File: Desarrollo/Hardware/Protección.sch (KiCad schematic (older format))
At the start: 46 parts, among them J1 Entradas Analógicas, U1 TPD2E001, U2 TPD2E001, U3 TPD2E001, U4 TPD2E001, U5 TPD2E001, U6 TPD2E001, U7 TPD2E001, U8 TPD2E001, U9 TPD2E001

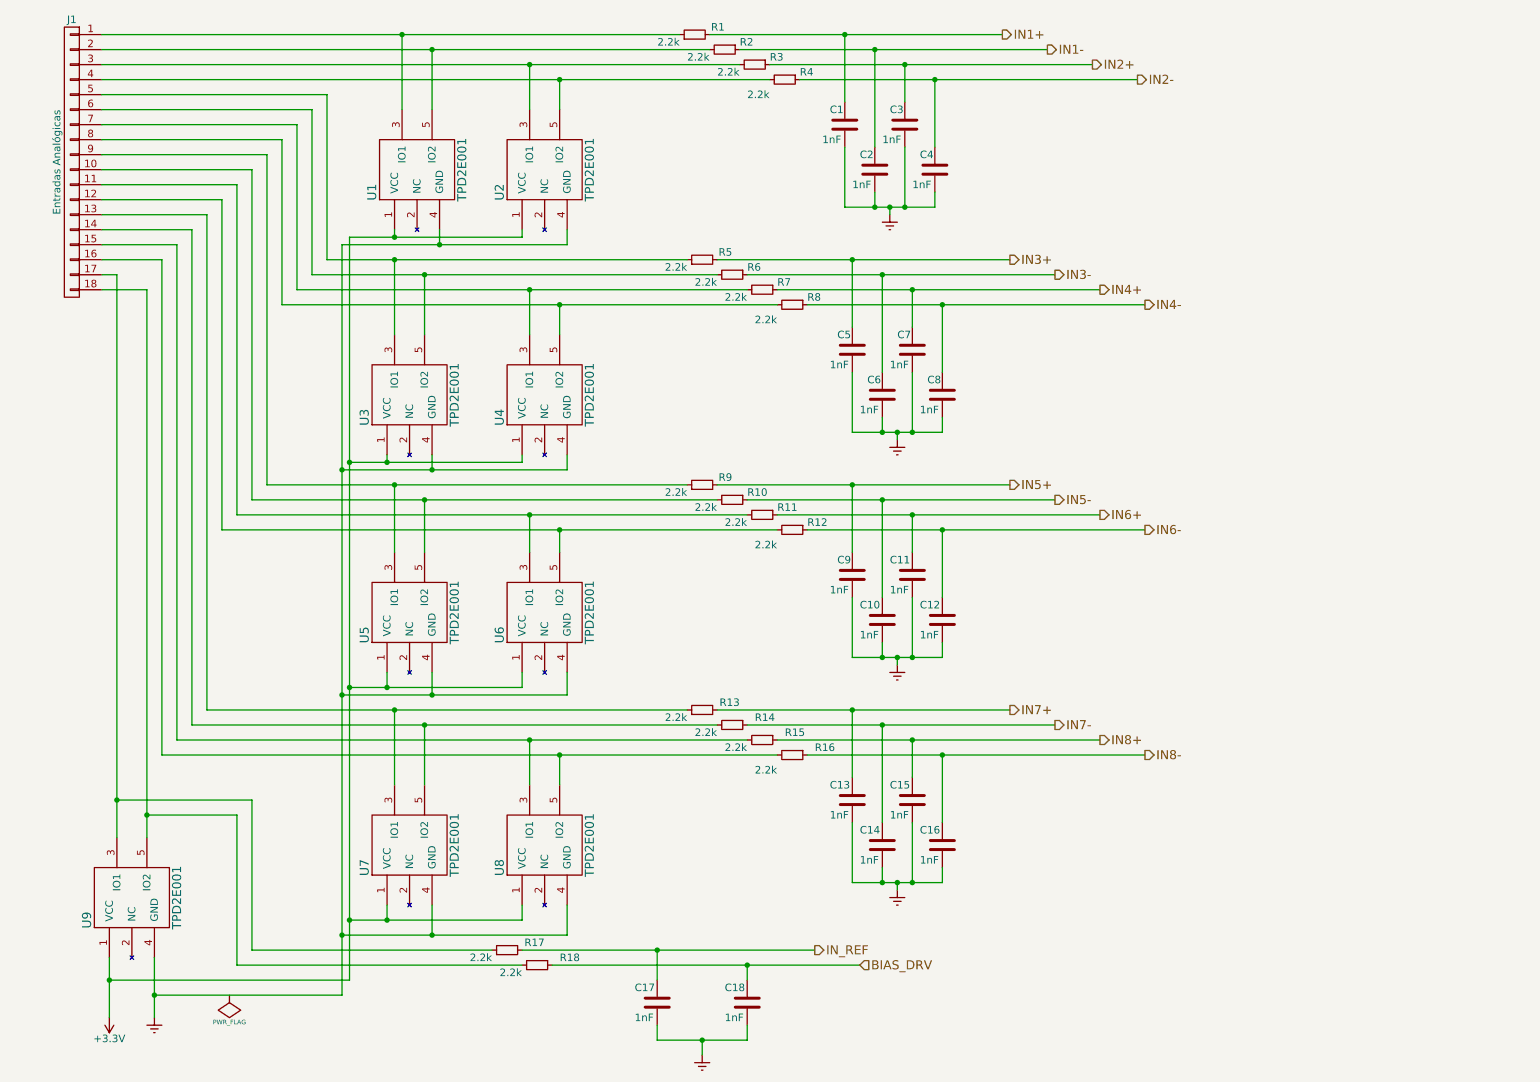
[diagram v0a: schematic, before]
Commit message: Finalización de primer ruteo estimado. Revisión de cantidad de v
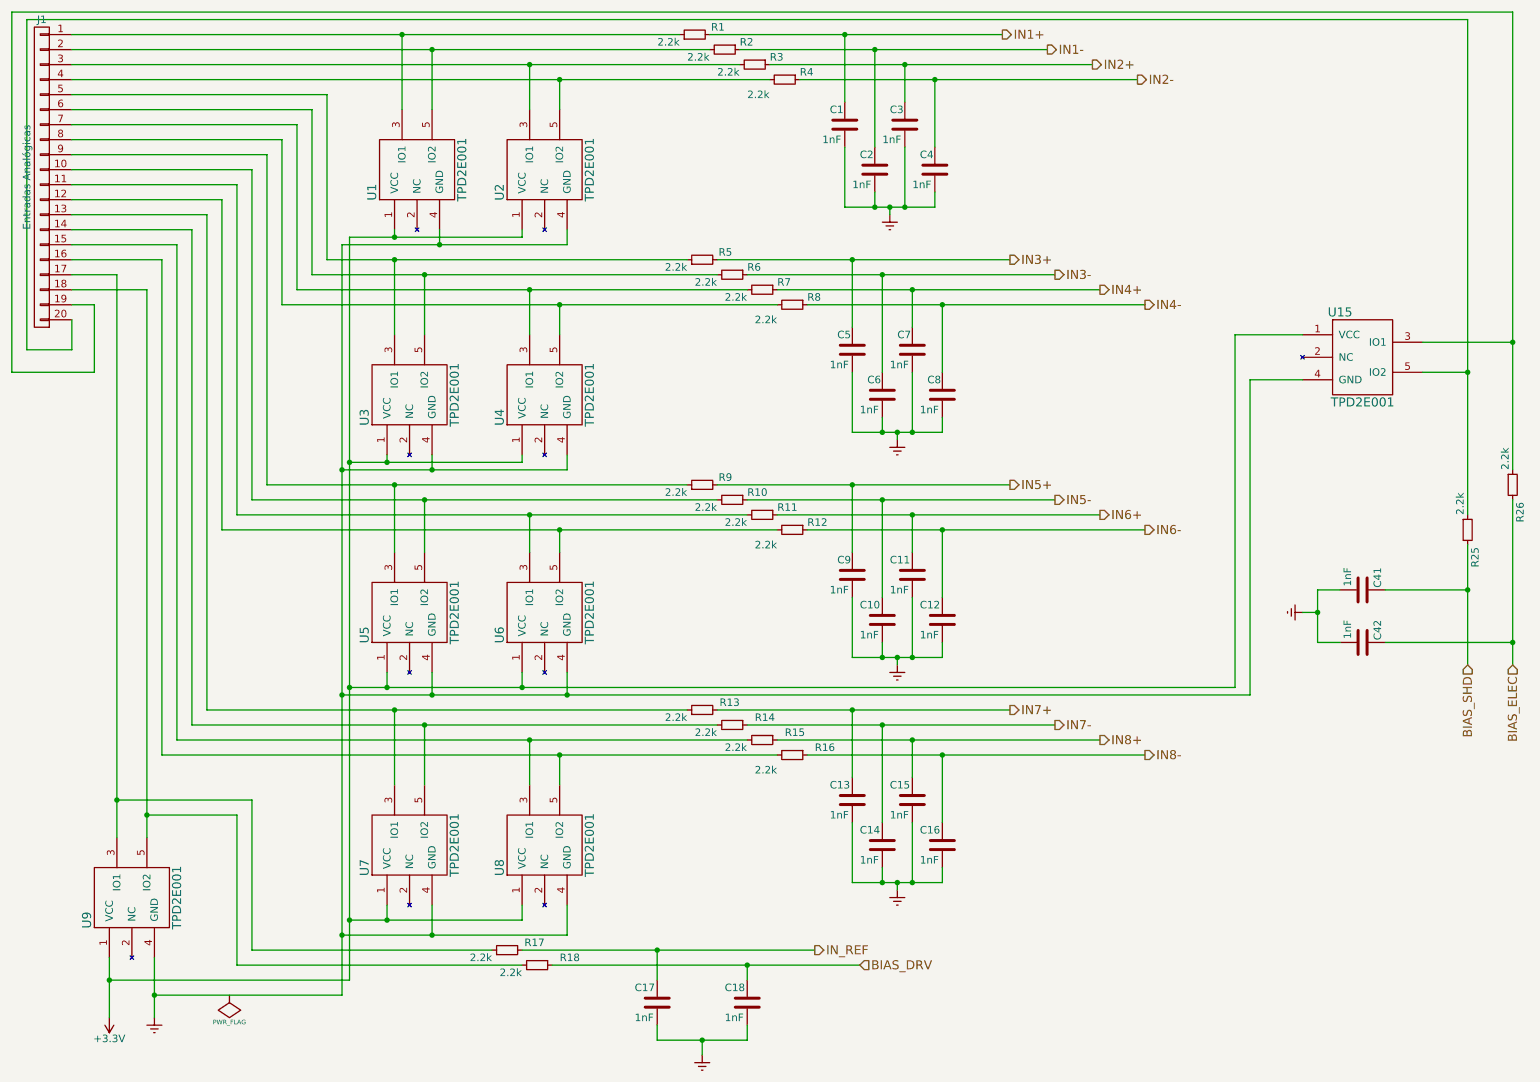
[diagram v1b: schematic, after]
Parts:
- removed J1: Entradas Analógicas, Pin_Headers:Pin_Header_Straight_1x18, symbol CONN_01X18
- added C41, C42: 1nF, Capacitors_SMD:C_0805, symbol C
- added J1: Entradas Analógicas, Pin_Headers:Pin_Header_Straight_1x20, symbol CONN_01X20
- added R25, R26: 2.2k, Resistors_SMD:R_0805, symbol R_Small
- added U15: TPD2E001, TO_SOT_Packages_SMD:SOT-23-5, symbol TPD2E001
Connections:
- net +3V3: now also U15.1 (VCC)
- net Earth: now also C41.2, C42.2, U15.4 (GND)
- net at R1.1, U1.3 (IO1): now also J1.1 (P1)
- net at R10.2, U5.5 (IO2): now also J1.10 (P10)
- net at R11.2, U6.3 (IO1): now also J1.11 (P11)
- net at R12.2, U6.5 (IO2): now also J1.12 (P12)
- net at R13.1, U7.3 (IO1): now also J1.13 (P13)
- net at R14.2, U7.5 (IO2): now also J1.14 (P14)
- net at R15.2, U8.3 (IO1): now also J1.15 (P15)
- net at R16.2, U8.5 (IO2): now also J1.16 (P16)
- net at R17.1, U9.3 (IO1): now also J1.17 (P17)
- net at R18.2, U9.5 (IO2): now also J1.18 (P18)
- net at R2.2, U1.5 (IO2): now also J1.2 (P2)
- net at R3.2, U2.3 (IO1): now also J1.3 (P3)
- net at R4.2, U2.5 (IO2): now also J1.4 (P4)
- net at R5.1, U3.3 (IO1): now also J1.5 (P5)
- net at R6.2, U3.5 (IO2): now also J1.6 (P6)
- net at R7.2, U4.3 (IO1): now also J1.7 (P7)
- net at R8.2, U4.5 (IO2): now also J1.8 (P8)
- net at R9.1, U5.3 (IO1): now also J1.9 (P9)
- new net: J1.19 (P19), R26.1, U15.3 (IO1)
- new net: J1.20 (P20), R25.1, U15.5 (IO2)
- new net BIAS_ELEC: C42.1, R26.2
- new net BIAS_SHD: C41.1, R25.2
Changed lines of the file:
@@
 encoding utf-8
 Sheet 2 4
-Title ""
+Title "Entradas Analógicas y Protección"
 Date ""
-Rev ""
-Comp ""
+Rev "1.0"
+Comp "Bruno Javier Cesario"
 Comment1 ""
 Comment2 ""
@@
 Comment4 ""
 $EndDescr
-$Comp
-L CONN_01X18 J1
-U 1 1 57BF0F9F
-P 950 1550
-F 0 "J1" H 950 2500 50  0000 C CNN
-F 1 "Entradas Analógicas" V 1050 1550 50  0000 C CNN
-F 2 "Pin_Headers:Pin_Header_Straight_1x18" H 950 1550 50  0001 C CNN
-F 3 "" H 950 1550 50  0000 C CNN
-	1    950  1550
-	-1   0    0    -1
-$EndComp
 $Comp
 L R_Small R1
@@
 $EndComp
 Wire Wire Line
-	2650 2200 2650 1100
-Wire Wire Line
-	2650 1100 1150 1100
-Wire Wire Line
-	1150 1200 2550 1200
+	2650 1100 2650 2200
+Wire Wire Line
+	950  1100 2650 1100
+Wire Wire Line
+	950  1200 2550 1200
 Wire Wire Line
 	2550 1200 2550 2300
 Wire Wire Line
-	2450 2400 2450 1300
-Wire Wire Line
-	2450 1300 1150 1300
-Wire Wire Line
-	1150 1400 2350 1400
+	2450 1300 2450 2400
+Wire Wire Line
+	950  1300 2450 1300
+Wire Wire Line
+	950  1400 2350 1400
 Wire Wire Line
 	2350 1400 2350 2500
 Wire Wire Line
-	1150 1500 2250 1500
+	950  1500 2250 1500
 Wire Wire Line
 	2250 1500 2250 3700
 Wire Wire Line
-	2150 3800 2150 1600
-Wire Wire Line
-	2150 1600 1150 1600
-Wire Wire Line
-	1150 1700 2050 1700
+	2150 1600 2150 3800
+Wire Wire Line
+	950  1600 2150 1600
+Wire Wire Line
+	950  1700 2050 1700
 Wire Wire Line
 	2050 1700 2050 3900
 Wire Wire Line
-	1950 4000 1950 1800
-Wire Wire Line
-	1950 1800 1150 1800
+	1950 1800 1950 4000
+Wire Wire Line
+	950  1800 1950 1800
 Wire Wire Line
 	1850 1900 1850 5200
 Wire Wire Line
-	1850 1900 1150 1900
-Wire Wire Line
-	1150 2000 1750 2000
+	950  1900 1850 1900
+Wire Wire Line
+	950  2000 1750 2000
 Wire Wire Line
 	1750 2000 1750 5300
@@
 	1650 2100 1650 5400
 Wire Wire Line
-	1650 2100 1150 2100
-Wire Wire Line
-	1150 2200 1550 2200
+	950  2100 1650 2100
+Wire Wire Line
+	950  2200 1550 2200
 Wire Wire Line
 	1550 2200 1550 5500
 Wire Wire Line
-	1150 2300 1250 2300
+	950  2300 1250 2300
 Wire Wire Line
 	1250 2300 1250 6050
 Wire Wire Line
-	1150 2400 1450 2400
+	950  2400 1450 2400
 Wire Wire Line
 	1450 2400 1450 6050
@@
 Connection ~ 5150 7400
 Wire Wire Line
-	1150 700  5000 700
-Wire Wire Line
-	1150 800  5200 800
-Wire Wire Line
-	1150 900  5400 900
-Wire Wire Line
-	1150 1000 5600 1000
+	950  700  5000 700
+Wire Wire Line
+	950  800  5200 800
+Wire Wire Line
+	950  900  5400 900
+Wire Wire Line
+	950  1000 5600 1000
 Wire Wire Line
 	3150 1200 3150 700
@@
 	3050 4950 3050 5050
 Wire Wire Line
-	2800 5050 3950 5050
+	2800 5050 8700 5050
 Wire Wire Line
 	3950 5050 3950 4950
@@
 	3350 4950 3350 5100
 Wire Wire Line
-	2750 5100 4250 5100
+	2750 5100 8800 5100
 Wire Wire Line
 	4250 5100 4250 4950
@@
 	-1   0    0    1
 $EndComp
+$Comp
+L TPD2E001 U15
+U 1 1 57D06AC4
+P 9550 2850
+F 0 "U15" H 9400 3150 60  0000 C CNN
+F 1 "TPD2E001" H 9550 2550 60  0000 C CNN
+F 2 "TO_SOT_Packages_SMD:SOT-23-5" H 9550 2850 60  0001 C CNN
+F 3 "" H 9550 2850 60  0000 C CNN
+	1    9550 2850
+	1    0    0    -1
+$EndComp
+$Comp
+L R_Small R26
+U 1 1 57D06E46
+P 10550 3700
+F 0 "R26" V 10600 3450 50  0000 L CNN
+F 1 "2.2k" V 10500 3800 50  0000 L CNN
+F 2 "Resistors_SMD:R_0805" H 10550 3700 50  0001 C CNN
+F 3 "" H 10550 3700 50  0000 C CNN
+	1    10550 3700
+	1    0    0    -1
+$EndComp
+$Comp
+L R_Small R25
+U 1 1 57D0710C
+P 10250 4000
+F 0 "R25" V 10300 3750 50  0000 L CNN
+F 1 "2.2k" V 10200 4100 50  0000 L CNN
+F 2 "Resistors_SMD:R_0805" H 10250 4000 50  0001 C CNN
+F 3 "" H 10250 4000 50  0000 C CNN
+	1    10250 4000
+	1    0    0    -1
+$EndComp
+$Comp
+L C C41
+U 1 1 57D079C5
+P 9550 4400
+F 0 "C41" H 9400 4500 50  0000 L CNN
+F 1 "1nF" H 9400 4300 50  0000 L CNN
+F 2 "Capacitors_SMD:C_0805" H 9588 4250 50  0001 C CNN
+F 3 "" H 9550 4400 50  0000 C CNN
+	1    9550 4400
+	0    1    1    0
+$EndComp
+$Comp
+L C C42
+U 1 1 57D07AE3
+P 9550 4750
+F 0 "C42" H 9400 4850 50  0000 L CNN
+F 1 "1nF" H 9400 4650 50  0000 L CNN
+F 2 "Capacitors_SMD:C_0805" H 9588 4600 50  0001 C CNN
+F 3 "" H 9550 4750 50  0000 C CNN
+	1    9550 4750
+	0    1    1    0
+$EndComp
+Wire Wire Line
+	9950 2950 10250 2950
+Wire Wire Line
+	10250 600  10250 3900
+Wire Wire Line
+	10250 4100 10250 4900
+Wire Wire Line
+	10250 4400 9700 4400
+Wire Wire Line
+	9700 4750 10550 4750
+Wire Wire Line
+	10550 3800 10550 4900
+Wire Wire Line
+	10550 550  10550 3600
+Wire Wire Line
+	10550 2750 9950 2750
+Wire Wire Line
+	8700 5050 8700 2700
+Wire Wire Line
+	8700 2700 9150 2700
+Connection ~ 3950 5050
+Wire Wire Line
+	9150 3000 8800 3000
+Wire Wire Line
+	8800 3000 8800 5100
+Connection ~ 4250 5100
+$Comp
+L Earth #PWR09
+U 1 1 57D08E33
+P 9150 4550
+F 0 "#PWR09" H 9150 4300 50  0001 C CNN
+F 1 "Earth" H 9150 4400 50  0001 C CNN
+F 2 "" H 9150 4550 50  0000 C CNN
+F 3 "" H 9150 4550 50  0000 C CNN
+	1    9150 4550
+	0    1    1    0
+$EndComp
+Wire Wire Line
+	9150 4550 9250 4550
+Wire Wire Line
+	9250 4400 9250 4750
+Wire Wire Line
+	9250 4400 9400 4400
+Wire Wire Line
+	9250 4750 9400 4750
+Connection ~ 9250 4550
+Text HLabel 10250 4900 3    60   Input ~ 0
+BIAS_SHD
+Text HLabel 10550 4900 3    60   Input ~ 0
+BIAS_ELEC
+Connection ~ 10250 4400
+Connection ~ 10550 4750
+Connection ~ 10250 2950
+Connection ~ 10550 2750
+$Comp
+L CONN_01X20 J1
+U 1 1 57D115B1
+P 750 1650
+F 0 "J1" H 750 2700 50  0000 C CNN
+F 1 "Entradas Analógicas" V 850 1650 50  0000 C CNN
+F 2 "Pin_Headers:Pin_Header_Straight_1x20" H 750 1650 60  0001 C CNN
+F 3 "" H 750 1650 60  0000 C CNN
+	1    750  1650
+	-1   0    0    -1
+$EndComp
+Wire Wire Line
+	950  2500 1100 2500
+Wire Wire Line
+	1100 2500 1100 2950
+Wire Wire Line
+	950  2600 950  2800
+Wire Wire Line
+	10250 600  650  600
+Wire Wire Line
+	650  600  650  2800
+Wire Wire Line
+	650  2800 950  2800
+Wire Wire Line
+	1100 2950 550  2950
+Wire Wire Line
+	550  2950 550  550
+Wire Wire Line
+	550  550  10550 550
 $EndSCHEMATC
